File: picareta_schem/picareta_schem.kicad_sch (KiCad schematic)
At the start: 16 parts, among them M1 Motor_DC, M2 Motor_DC, M3 Motor_DC

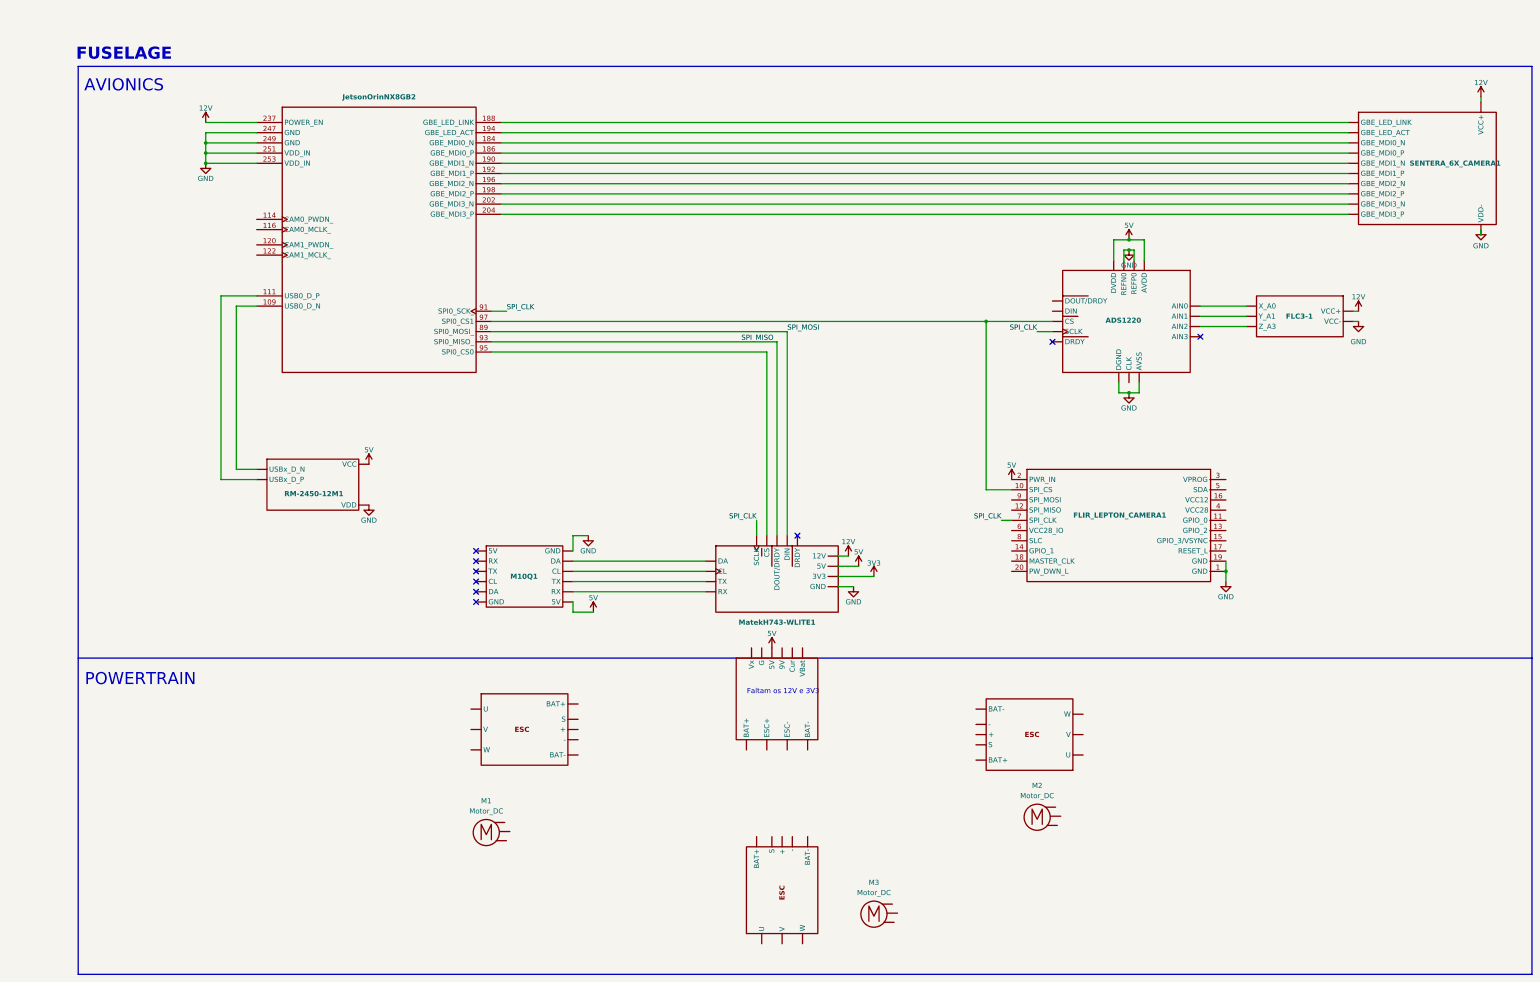
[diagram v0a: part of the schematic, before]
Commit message: Lowkirkenuily Good Avionics Schematic
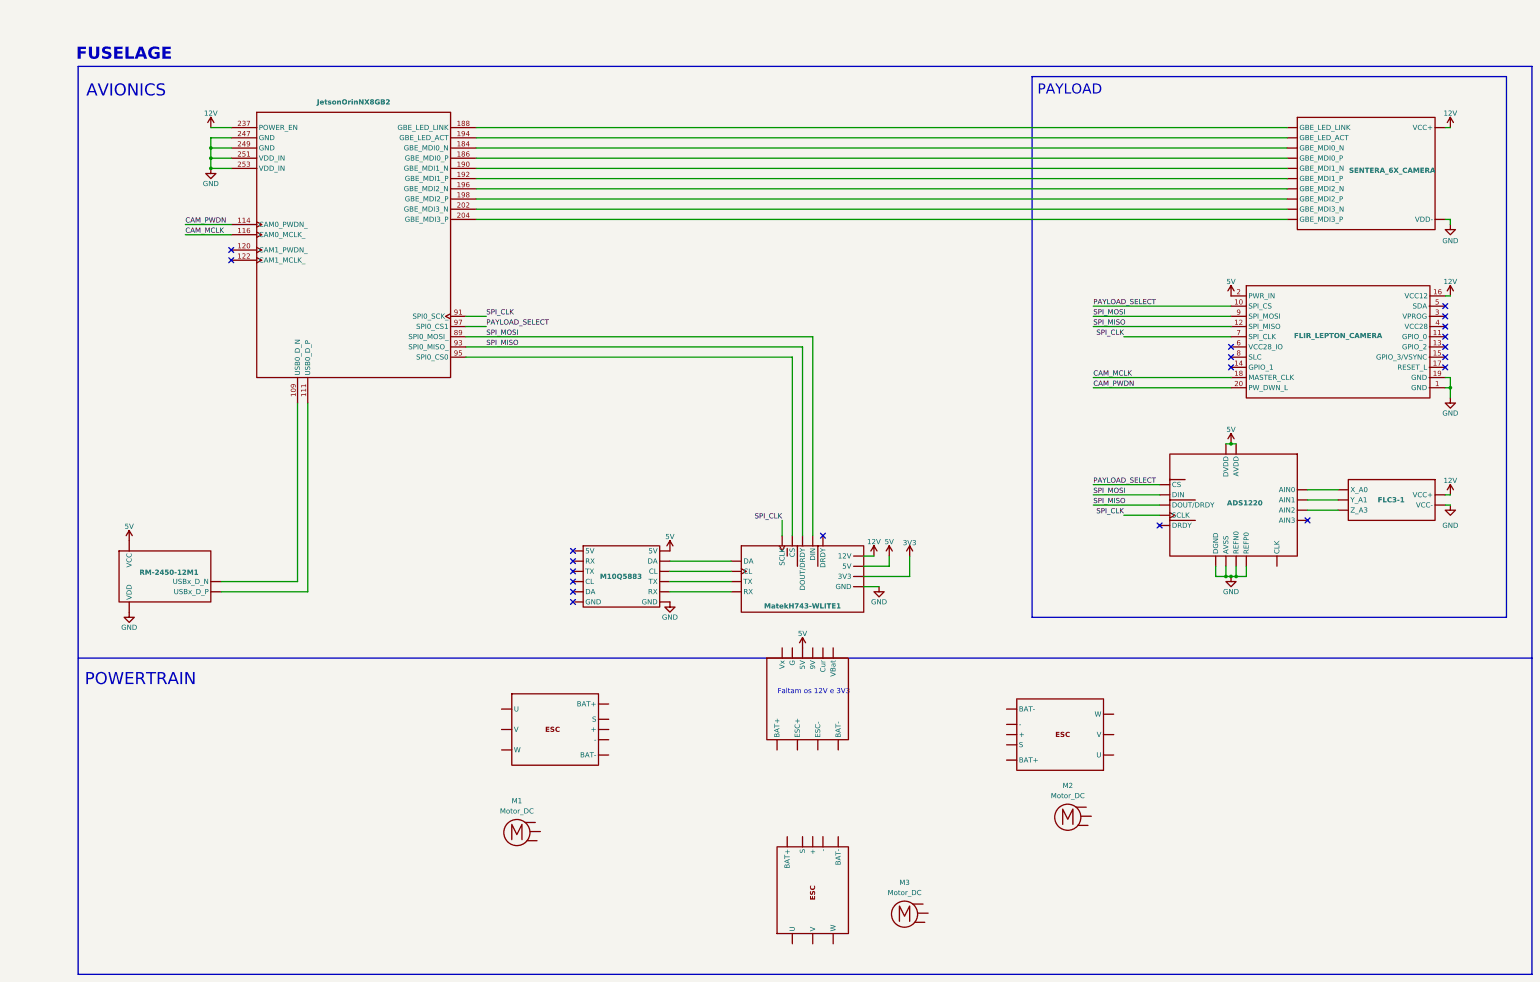
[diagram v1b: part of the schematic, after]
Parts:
- removed FLIR_LEPTON_CAMERA1: (no value), symbol Library_Laura_PIC:FLIR_Lepton_250-0577-00_DS_1-2021
- removed M10Q1: (no value), symbol Library_Laura_PIC:M10Q5883
- removed SENTERA_6X_CAMERA1: (no value), symbol Library_Laura_PIC:SENTERA_6X_CAMERA
- added FLIR_LEPTON_CAMERA: (no value), symbol Library_Laura_PIC:FLIR_Lepton_250-0577-00_DS_1-2021
- added M10Q5883: (no value), symbol Library_Laura_PIC:M10Q5883
- added SENTERA_6X_CAMERA: (no value), symbol Library_Laura_PIC:SENTERA_6X_CAMERA
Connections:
- net 12V: now also FLIR_LEPTON_CAMERA.16 (VCC12), SENTERA_6X_CAMERA. (VDD-)
- net 5V: now also FLIR_LEPTON_CAMERA.2 (PWR_IN), M10Q5883. (GND)
- net GND: now also FLIR_LEPTON_CAMERA.1 (GND), FLIR_LEPTON_CAMERA.19 (GND), M10Q5883. (GND), SENTERA_6X_CAMERA. (VDD-)
- net SPI_CLK: now also FLIR_LEPTON_CAMERA.7 (SPI_CLK)
- net SPI_MISO: now also ADS1220. (AIN3), FLIR_LEPTON_CAMERA.12 (SPI_MISO)
- net SPI_MOSI: now also ADS1220. (AIN3), FLIR_LEPTON_CAMERA.9 (SPI_MOSI)
- net PAYLOAD_SELECT: now reaches ADS1220. (AIN3), JetsonOrinNX8GB2.97 (SPI0_CS1)
- net PAYLOAD_SELECT: now also FLIR_LEPTON_CAMERA.10 (SPI_CS)
- net CAM_PWDN: now reaches JetsonOrinNX8GB2.114 (CAM0_PWDN_)
- net CAM_PWDN: now also FLIR_LEPTON_CAMERA.20 (PW_DWN_L)
- net CAM_MCLK: now reaches JetsonOrinNX8GB2.116 (CAM0_MCLK_)
- net CAM_MCLK: now also FLIR_LEPTON_CAMERA.18 (MASTER_CLK)
- net at JetsonOrinNX8GB2.184 (GBE_MDI0_N): now also SENTERA_6X_CAMERA. (VDD-)
- net at JetsonOrinNX8GB2.186 (GBE_MDI0_P): now also SENTERA_6X_CAMERA. (VDD-)
- net at JetsonOrinNX8GB2.188 (GBE_LED_LINK): now also SENTERA_6X_CAMERA. (VDD-)
- net at JetsonOrinNX8GB2.190 (GBE_MDI1_N): now also SENTERA_6X_CAMERA. (VDD-)
- net at JetsonOrinNX8GB2.192 (GBE_MDI1_P): now also SENTERA_6X_CAMERA. (VDD-)
- net at JetsonOrinNX8GB2.194 (GBE_LED_ACT): now also SENTERA_6X_CAMERA. (VDD-)
- net at JetsonOrinNX8GB2.196 (GBE_MDI2_N): now also SENTERA_6X_CAMERA. (VDD-)
- net at JetsonOrinNX8GB2.198 (GBE_MDI2_P): now also SENTERA_6X_CAMERA. (VDD-)
- net at JetsonOrinNX8GB2.202 (GBE_MDI3_N): now also SENTERA_6X_CAMERA. (VDD-)
- net at JetsonOrinNX8GB2.204 (GBE_MDI3_P): now also SENTERA_6X_CAMERA. (VDD-)
- new net: ADS1220. (AIN3), FLC3-1. (Z_A3) (x3)
- new net: M10Q5883. (GND), MatekH743-WLITE1. (GND) (x4)
- no-connect marks 9 -> 21
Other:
- note added: "PAYLOAD"
- moved on the sheet: FLC3-1, M1, M2, M3, MatekH743-WLITE1
